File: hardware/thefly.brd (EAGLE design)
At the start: 54 x 54 mm, 40 parts, among them IC1 AP7313-1.8, J1 54-00298-HOLES, U1 SGTL5000XNLA3, U2 MAX4466EXK

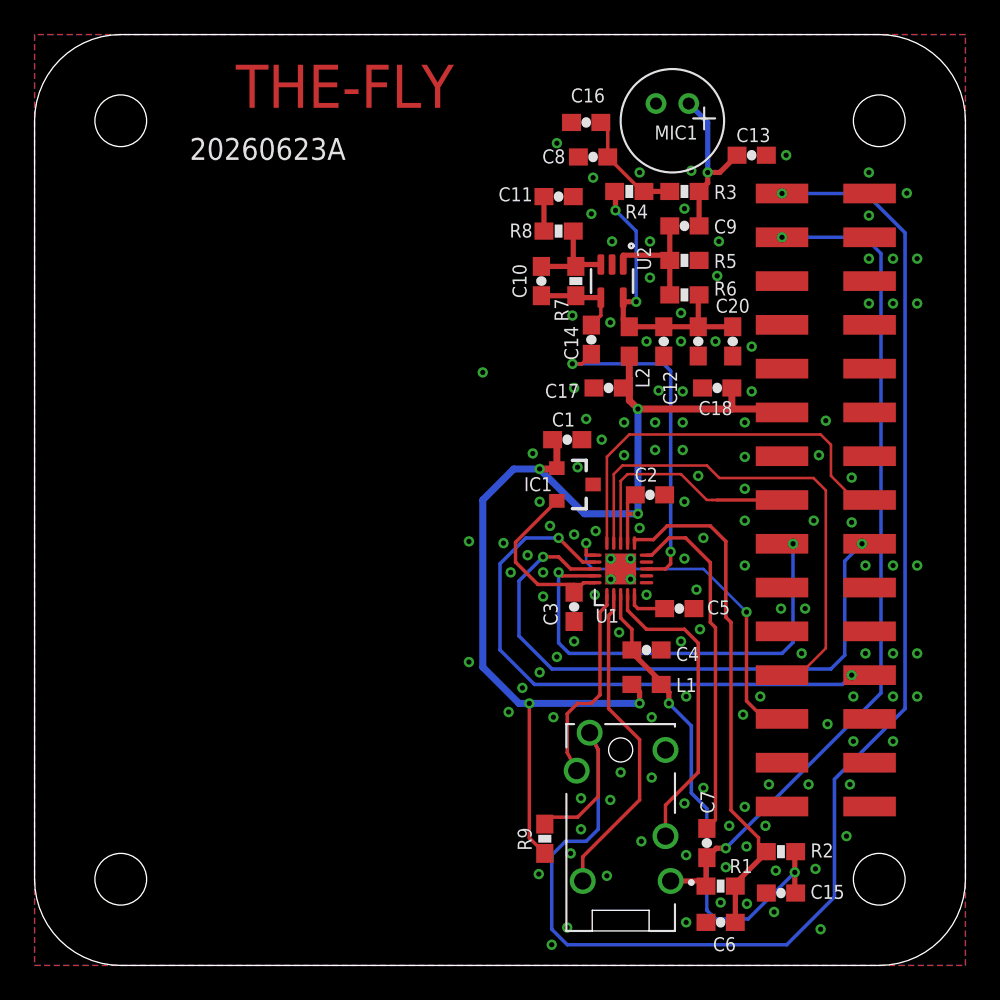
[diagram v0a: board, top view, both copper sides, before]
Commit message: pcb layout change
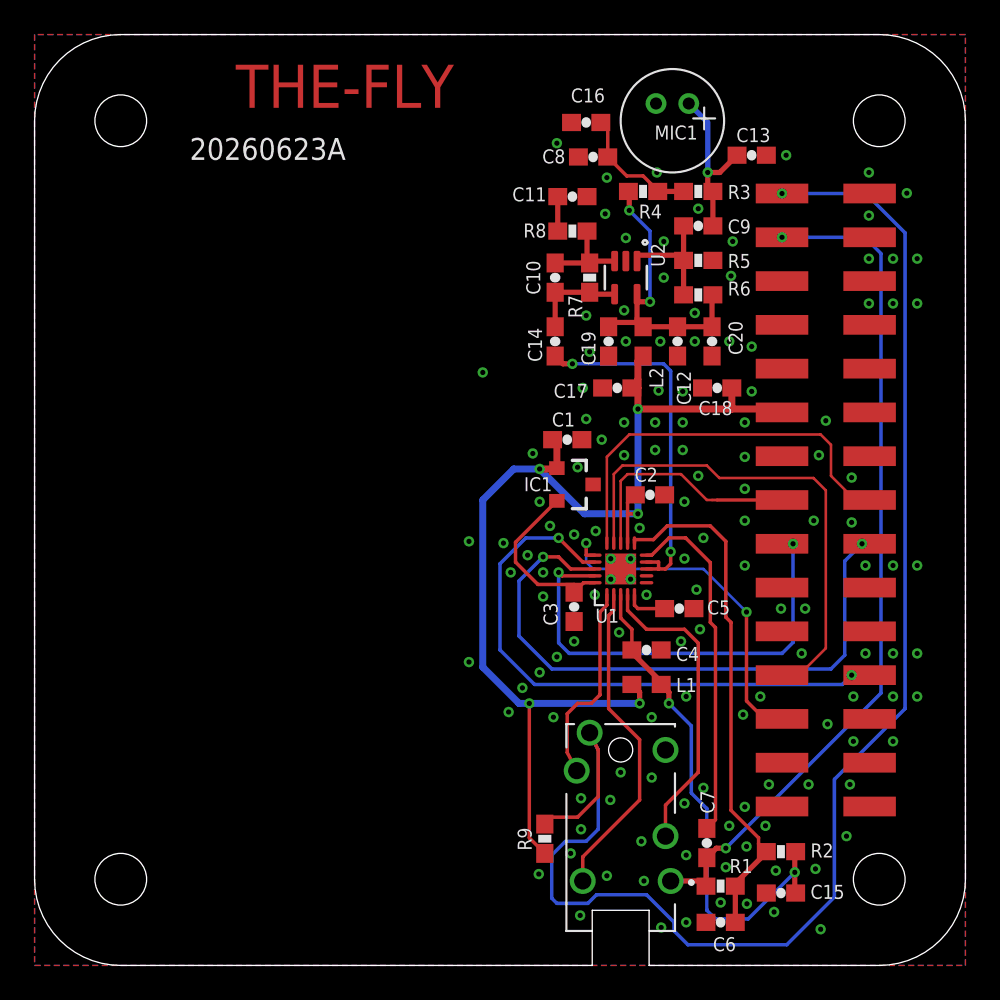
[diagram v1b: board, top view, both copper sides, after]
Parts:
- moved C19 5.20 mm to (33.3, 36.2)
- moved C14 2.10 mm to (30.2, 36.2)
- moved C20 1.20 mm to (39.3, 36.2)
- moved R7 0.82 mm to (32.2, 39.9)
- moved C10 0.82 mm to (30.2, 39.9)
- moved U2 0.82 mm to (34.3, 39.9)
- moved C11 0.80 mm to (31.2, 44.6)
- moved R8 0.80 mm to (31.2, 42.6)
- moved C12 0.80 mm to (37.3, 36.2)
- moved C9 0.80 mm to (38.5, 42.9)
- moved L2 0.80 mm to (35.3, 36.2)
- moved R3 0.80 mm to (38.5, 44.9)
- moved R4 0.80 mm to (35.3, 44.9)
- moved R5 0.80 mm to (38.5, 40.9)
- moved R6 0.80 mm to (38.5, 38.9)
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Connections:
- net MIC2: now also U1.9
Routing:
- net MIC2: track 19.9 -> 20.9 mm
- net N$11: track 6.59 -> 7.42 mm
- net VCCA2: track 17.7 -> 18.4 mm
- net GND: vias 134 -> 136
